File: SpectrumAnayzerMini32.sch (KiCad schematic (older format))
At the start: 519 parts, among them J1 Input, J2 Output

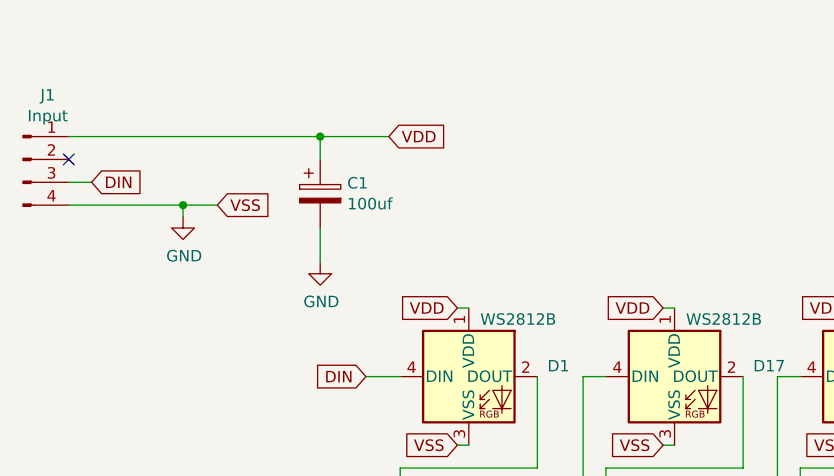
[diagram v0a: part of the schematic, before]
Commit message: shrink the board
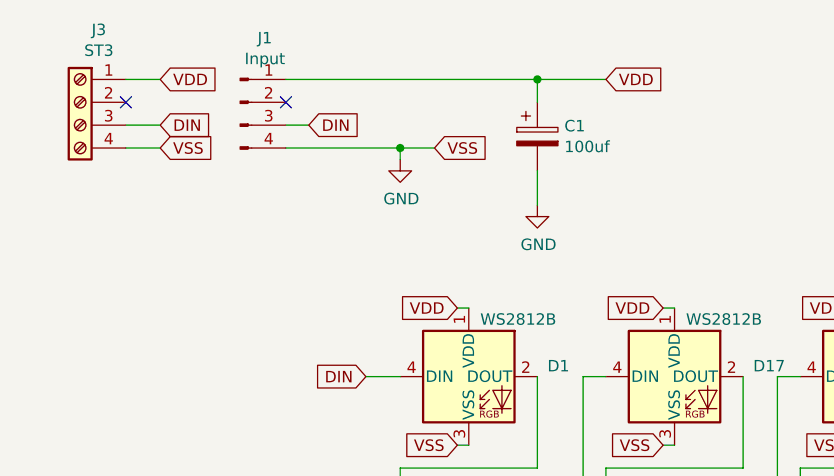
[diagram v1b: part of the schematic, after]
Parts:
- added J3: ST3, TerminalBlock_Phoenix:TerminalBlock_Phoenix_MPT-0,5-4-2.54_1x04_P2.54mm_Horizontal, symbol Connector:Screw_Terminal_01x04
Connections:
- net DIN: now also J3.3 (Pin_3)
- net GND: now also J3.4 (Pin_4)
- net VDD: now also J3.1 (Pin_1)
- no-connect marks 2 -> 3
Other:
- moved on the sheet: C1, J1
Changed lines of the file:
@@
 L power:GND #PWR01
 U 1 1 5E187269
-P 1250 1450
-F 0 "#PWR01" H 1250 1200 50  0001 C CNN
-F 1 "GND" H 1255 1277 50  0000 C CNN
-F 2 "" H 1250 1450 50  0001 C CNN
-F 3 "" H 1250 1450 50  0001 C CNN
-	1    1250 1450
+P 2200 1200
+F 0 "#PWR01" H 2200 950 50  0001 C CNN
+F 1 "GND" H 2205 1027 50  0000 C CNN
+F 2 "" H 2200 1200 50  0001 C CNN
+F 3 "" H 2200 1200 50  0001 C CNN
+	1    2200 1200
 	1    0    0    -1
 $EndComp
@@
 	1    0    0    -1
 $EndComp
-Text GLabel 2150 1100 2    50   Input ~ 0
+Text GLabel 3100 850  2    50   Input ~ 0
 VDD
-Text GLabel 1400 1400 2    50   Input ~ 0
+Text GLabel 2350 1150 2    50   Input ~ 0
 VSS
 $Comp
 L Device:CP C1
 U 1 1 60C6F4E3
-P 1850 1350
-F 0 "C1" H 1968 1396 50  0000 L CNN
-F 1 "100uf" H 1968 1305 50  0000 L CNN
-F 2 "Capacitor_THT:CP_Radial_D5.0mm_P2.50mm" H 1888 1200 50  0001 C CNN
-F 3 "~" H 1850 1350 50  0001 C CNN
-	1    1850 1350
+P 2800 1100
+F 0 "C1" H 2918 1146 50  0000 L CNN
+F 1 "100uf" H 2918 1055 50  0000 L CNN
+F 2 "Capacitor_THT:CP_Radial_D5.0mm_P2.50mm" H 2838 950 50  0001 C CNN
+F 3 "~" H 2800 1100 50  0001 C CNN
+	1    2800 1100
 	1    0    0    -1
 $EndComp
@@
 L power:GND #PWR02
 U 1 1 60DFF3C3
-P 1850 1650
-F 0 "#PWR02" H 1850 1400 50  0001 C CNN
-F 1 "GND" H 1855 1477 50  0000 C CNN
-F 2 "" H 1850 1650 50  0001 C CNN
-F 3 "" H 1850 1650 50  0001 C CNN
-	1    1850 1650
+P 2800 1400
+F 0 "#PWR02" H 2800 1150 50  0001 C CNN
+F 1 "GND" H 2805 1227 50  0000 C CNN
+F 2 "" H 2800 1400 50  0001 C CNN
+F 3 "" H 2800 1400 50  0001 C CNN
+	1    2800 1400
 	1    0    0    -1
 $EndComp
 Wire Wire Line
-	1850 1650 1850 1500
+	2800 1400 2800 1250
 Wire Wire Line
-	750  1100 1850 1100
+	1700 850  2800 850
 Wire Wire Line
-	1850 1100 1850 1200
+	2800 850  2800 950
 Wire Wire Line
 	2050 2150 2200 2150
-Text GLabel 850  1300 2    50   Input ~ 0
+Text GLabel 1800 1050 2    50   Input ~ 0
 DIN
 Wire Wire Line
-	850  1300 750  1300
+	1800 1050 1700 1050
 Text GLabel 2050 2150 0    50   Input ~ 0
 DIN
 Wire Wire Line
-	1850 1100 2150 1100
-Connection ~ 1850 1100
+	2800 850  3100 850
+Connection ~ 2800 850
 Wire Wire Line
 	15150 2150 15150 2550
@@
 L Connector:Conn_01x04_Male J1
 U 1 1 60CA0B50
-P 550 1200
-F 0 "J1" H 658 1481 50  0000 C CNN
-F 1 "Input" H 658 1390 50  0000 C CNN
-F 2 "Connector_PinHeader_2.54mm:PinHeader_1x04_P2.54mm_Vertical" H 550 1200 50  0001 C CNN
-F 3 "~" H 550 1200 50  0001 C CNN
-	1    550  1200
+P 1500 950
+F 0 "J1" H 1608 1231 50  0000 C CNN
+F 1 "Input" H 1608 1140 50  0000 C CNN
+F 2 "Connector_PinHeader_2.54mm:PinHeader_1x04_P2.54mm_Vertical" H 1500 950 50  0001 C CNN
+F 3 "~" H 1500 950 50  0001 C CNN
+	1    1500 950
 	1    0    0    -1
 $EndComp
 Wire Wire Line
-	750  1400 1250 1400
+	1700 1150 2200 1150
 Wire Wire Line
-	1250 1450 1250 1400
-Connection ~ 1250 1400
+	2200 1200 2200 1150
+Connection ~ 2200 1150
 Wire Wire Line
-	1250 1400 1400 1400
-NoConn ~ 750  1200
+	2200 1150 2350 1150
+NoConn ~ 1700 950
 $Comp
 L Connector:Conn_01x04_Male J2
@@
 $EndComp
 NoConn ~ 30950 14500
+$Comp
+L Connector:Screw_Terminal_01x04 J3
+U 1 1 5EAF3C24
+P 800 950
+F 0 "J3" H 718 1267 50  0000 C CNN
+F 1 "ST3" H 718 1176 50  0000 C CNN
+F 2 "TerminalBlock_Phoenix:TerminalBlock_Phoenix_MPT-0,5-4-2.54_1x04_P2.54mm_Horizontal" H 800 950 50  0001 C CNN
+F 3 "~" H 800 950 50  0001 C CNN
+	1    800  950
+	-1   0    0    -1
+$EndComp
+Text GLabel 1150 1050 2    50   Input ~ 0
+DIN
+Text GLabel 1150 1150 2    50   Input ~ 0
+VSS
+Text GLabel 1150 850  2    50   Input ~ 0
+VDD
+NoConn ~ 1000 950
+Wire Wire Line
+	1000 1150 1150 1150
+Wire Wire Line
+	1000 1050 1150 1050
+Wire Wire Line
+	1000 850  1150 850
 $EndSCHEMATC
